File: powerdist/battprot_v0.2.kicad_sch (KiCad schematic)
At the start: 34 parts, among them Q22 L2N7002SLLT1G, Q23 SIS412DN, Q24 L2N7002SLLT1G, Q25 SIS412DN, SW9 JS202011CQN, U9 BQ7791508PWR

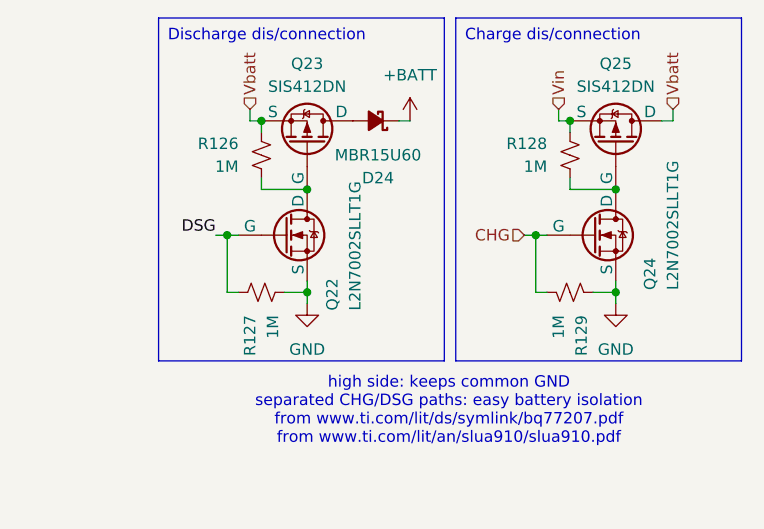
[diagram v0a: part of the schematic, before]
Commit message: lab 23/10
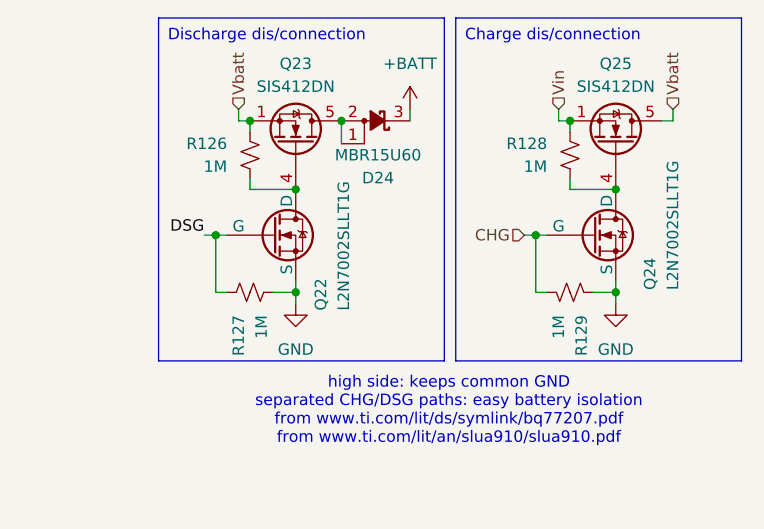
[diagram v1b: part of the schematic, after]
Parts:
- C100, C101, C102, C103, C104, C105, C106, C107, C108, C109: footprint (none) -> Capacitor_SMD:C_0603_1608Metric
- D24: symbol Device:D_Schottky_Small_Filled -> D_Schottky_AAK_Parallel_Small_Filled:D_Schottky_AAK
- Q22, Q24: footprint (none) -> Package_TO_SOT_SMD:SOT-23
- Q23, Q25: footprint (none) -> Package_SO:Vishay_PowerPAK_1212-8_Single; symbol Simulation_SPICE:PMOS -> Transistor_FET:SiS454DN
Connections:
- net +BATT: now also D24.3 (K); no longer D24.1 (K)
- net Vbatt: now also Q23.1 (S), Q23.2 (S), Q25.5 (D); no longer Q25.1 (D)
- net Vin: now also Q25.1 (S), Q25.2 (S)
- net at Q22.1 (D), R126.2: now also Q23.4 (G); no longer Q23.2 (G)
- net at Q24.1 (D), R128.2: now also Q25.4 (G); no longer Q25.2 (G)
- net at D24.2 (A): now also D24.1 (A), Q23.5 (D); no longer Q23.1 (D)
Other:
- moved on the sheet: Q22, Q23, R126, R127
